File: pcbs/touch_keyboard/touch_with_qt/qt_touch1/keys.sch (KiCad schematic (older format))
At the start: 28 parts

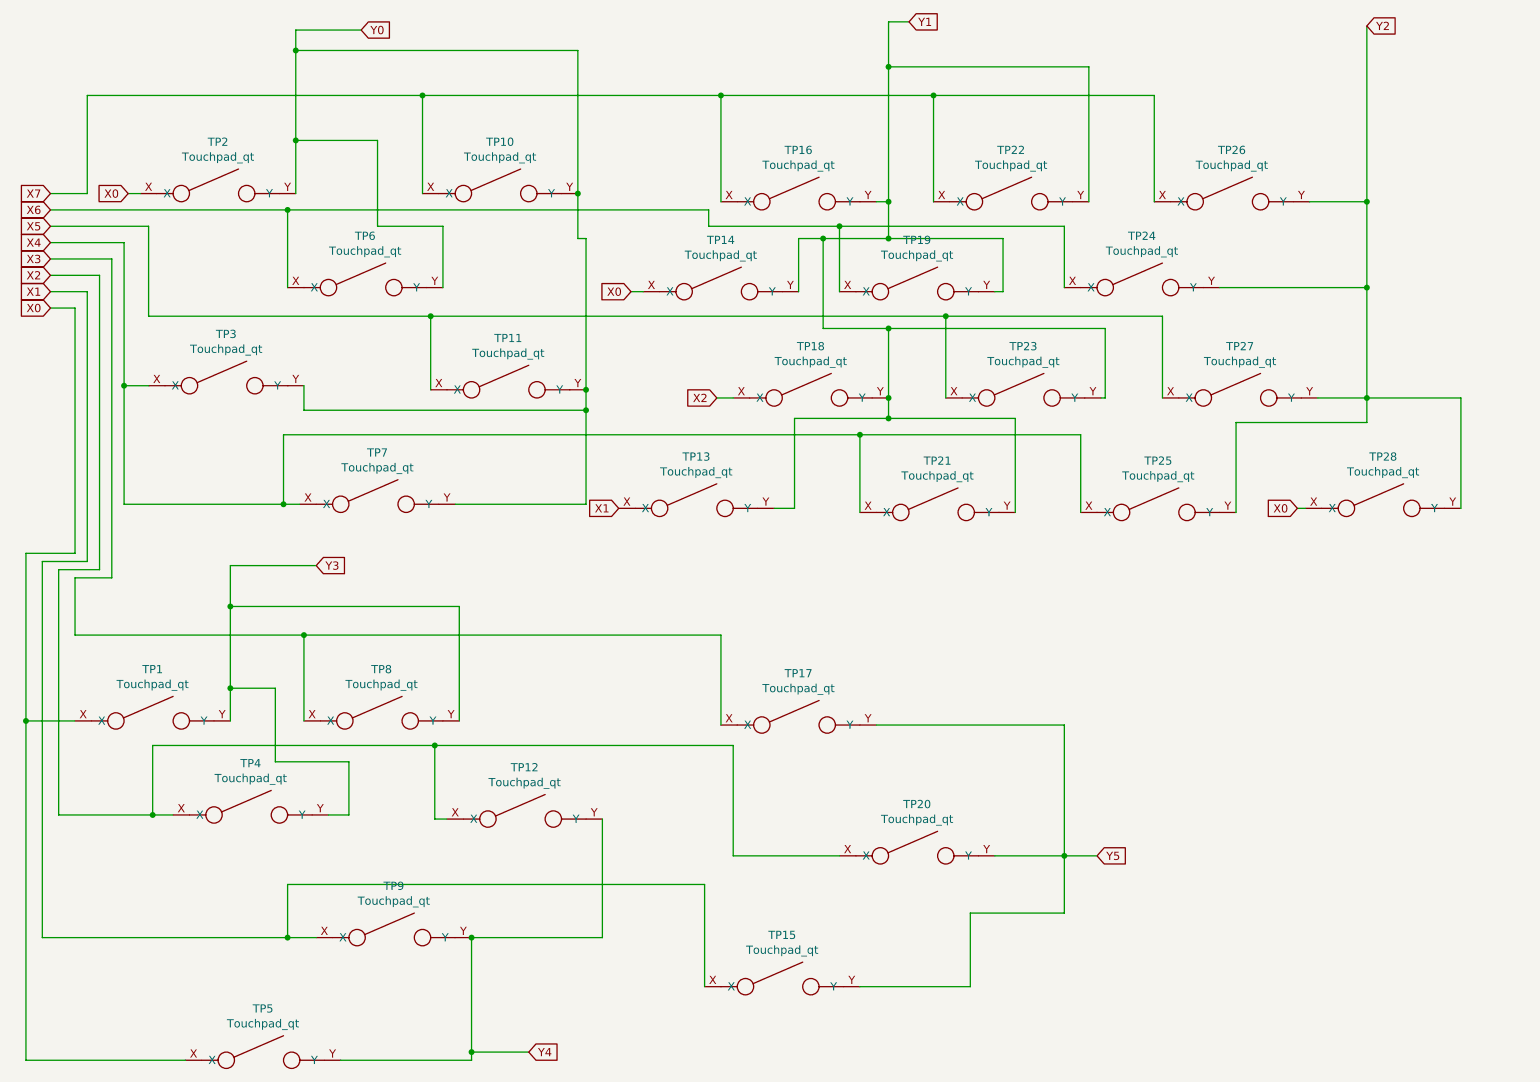
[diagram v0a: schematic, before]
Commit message: Updates
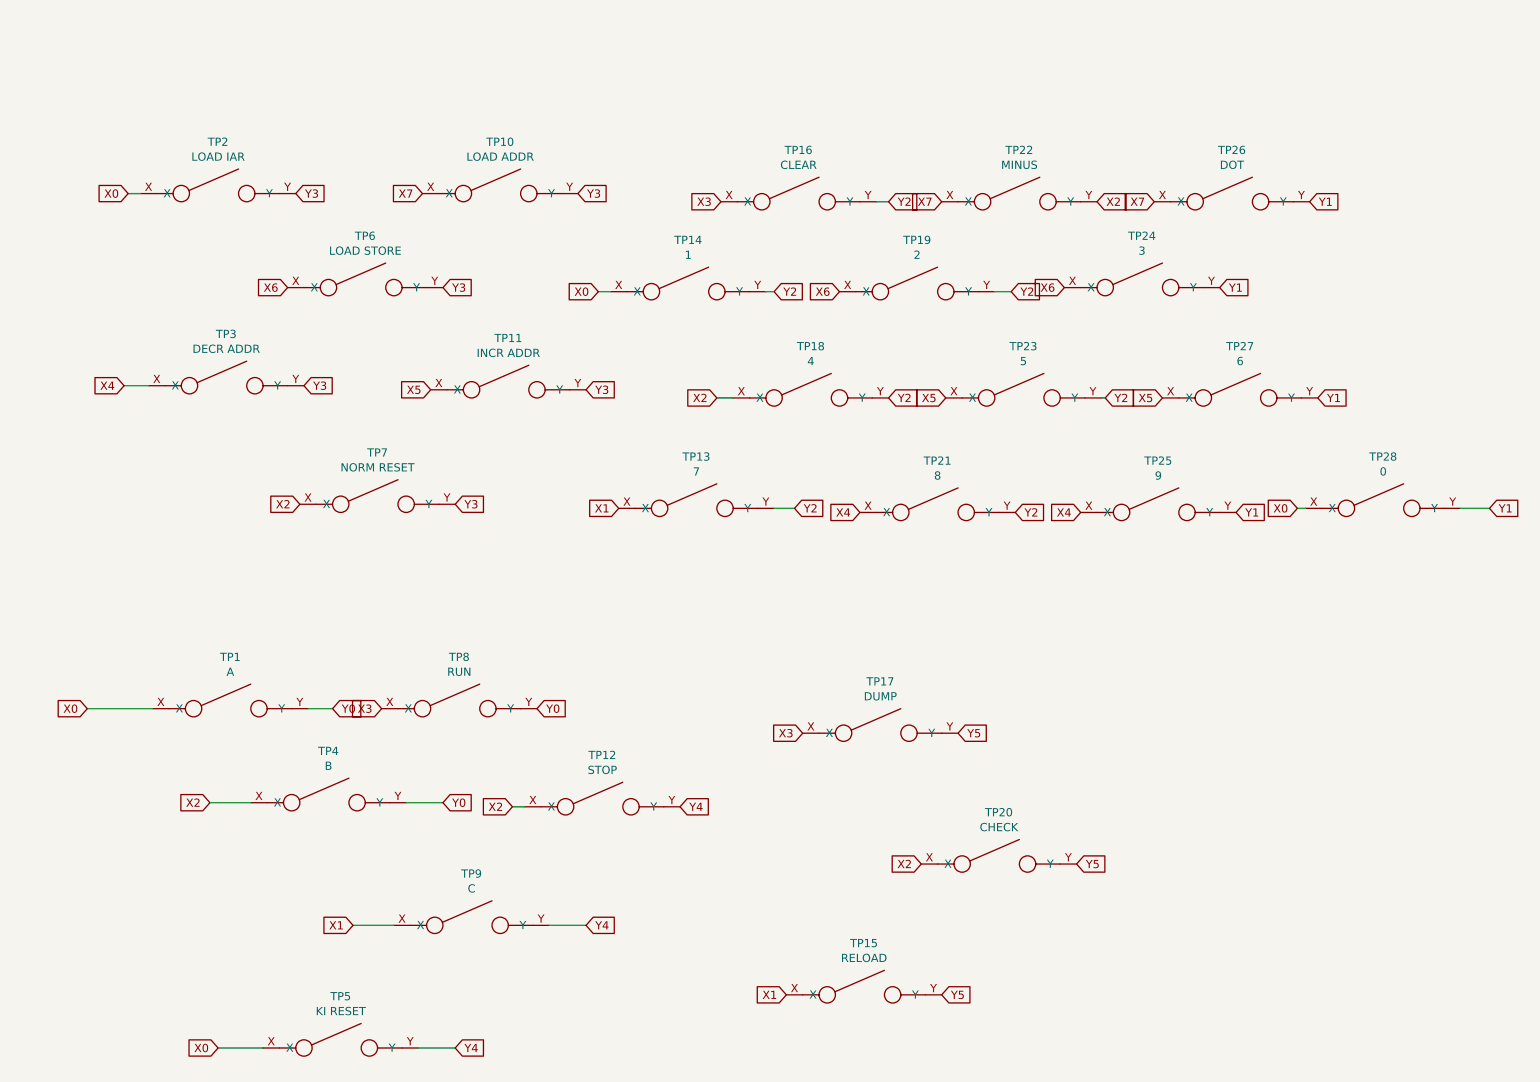
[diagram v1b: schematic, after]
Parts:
- TP1: value Touchpad_qt -> A
- TP10: value Touchpad_qt -> LOAD ADDR
- TP11: value Touchpad_qt -> INCR ADDR
- TP12: value Touchpad_qt -> STOP
- TP13: value Touchpad_qt -> 7
- TP14: value Touchpad_qt -> 1
- TP15: value Touchpad_qt -> RELOAD
- TP16: value Touchpad_qt -> CLEAR
- TP17: value Touchpad_qt -> DUMP
- TP18: value Touchpad_qt -> 4
- TP19: value Touchpad_qt -> 2
- TP2: value Touchpad_qt -> LOAD IAR
- TP20: value Touchpad_qt -> CHECK
- TP21: value Touchpad_qt -> 8
- TP22: value Touchpad_qt -> MINUS
- TP23: value Touchpad_qt -> 5
- TP24: value Touchpad_qt -> 3
- TP25: value Touchpad_qt -> 9
- TP26: value Touchpad_qt -> DOT
- TP27: value Touchpad_qt -> 6
- TP28: value Touchpad_qt -> 0
- TP3: value Touchpad_qt -> DECR ADDR
- TP4: value Touchpad_qt -> B
- TP5: value Touchpad_qt -> KI RESET
- TP6: value Touchpad_qt -> LOAD STORE
- TP7: value Touchpad_qt -> NORM RESET
- TP8: value Touchpad_qt -> RUN
- TP9: value Touchpad_qt -> C
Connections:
- net X2: now also TP22.Y, TP7.X
- net X3: now also TP16.X
- net X4: no longer TP7.X
- net X7: no longer TP16.X
- net Y0: now also TP1.Y, TP4.Y, TP8.Y; no longer TP10.Y, TP11.Y, TP2.Y, TP3.Y, TP6.Y, TP7.Y
- net Y1: now also TP24.Y, TP25.Y, TP26.Y, TP27.Y, TP28.Y; no longer TP13.Y, TP14.Y, TP16.Y, TP18.Y, TP19.Y, TP21.Y, TP22.Y, TP23.Y
- net Y2: now also TP13.Y, TP14.Y, TP16.Y, TP18.Y, TP19.Y, TP21.Y, TP23.Y; no longer TP24.Y, TP25.Y, TP26.Y, TP27.Y, TP28.Y
- net Y3: now also TP10.Y, TP11.Y, TP2.Y, TP3.Y, TP6.Y, TP7.Y; no longer TP1.Y, TP4.Y, TP8.Y
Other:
- moved on the sheet: TP1, TP12, TP14, TP15, TP17, TP20, TP22, TP4, TP5, TP8, TP9
